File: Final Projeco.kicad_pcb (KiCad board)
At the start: 6 copper layers, 26.5 x 45 mm, 26 parts, among them U1 ESP32-S3, U2 GT-USB-7004N, U3 NCP167BMX330TBG, U4 LY68L6400SLIT, U5 PTS830GG140SMTRLFS, U6 PTS830GG140SMTRLFS, U7 220S-2*16P_H=8_5MM_Ytype_L=3_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, X1 TZ1269D

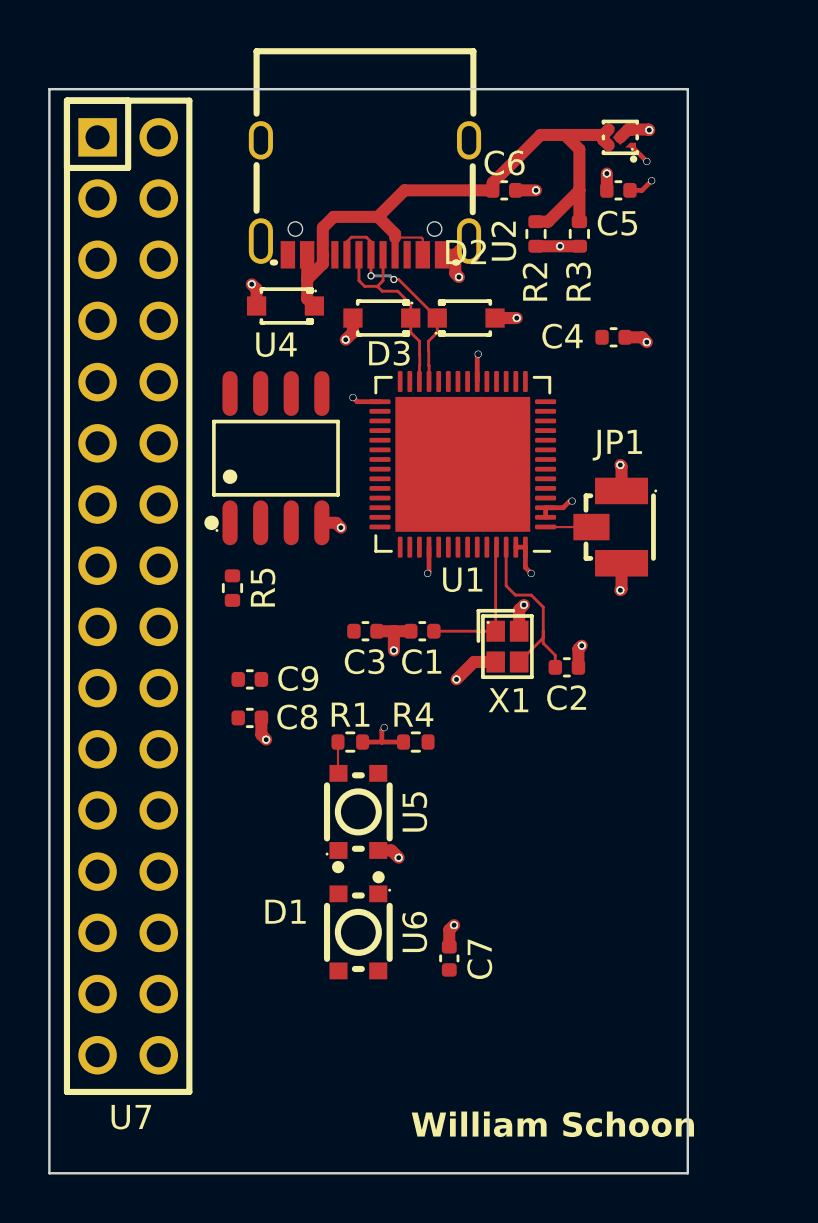
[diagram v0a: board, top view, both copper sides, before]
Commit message: stuff
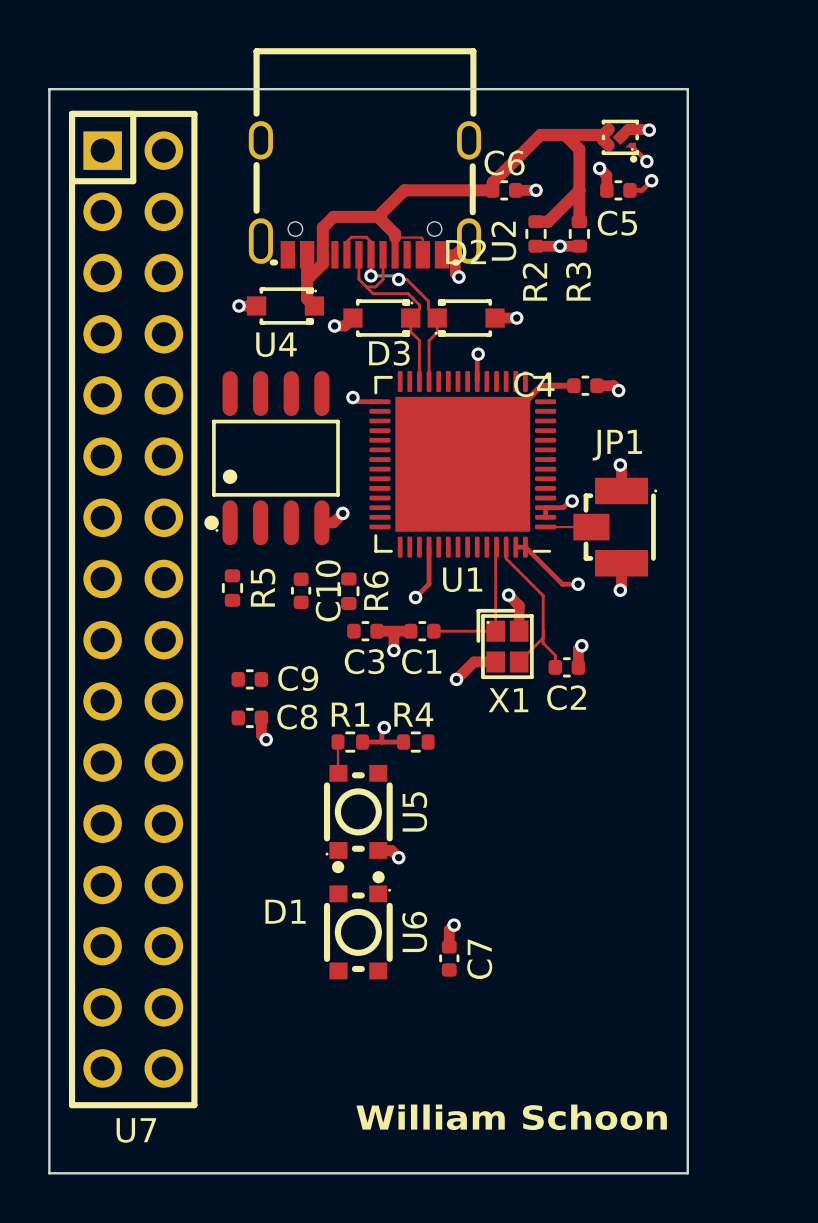
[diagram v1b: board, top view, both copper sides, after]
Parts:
- added C10: 1uF, Capacitor_SMD:C_0402_1005Metric, F.Cu at (35.5, 36.3)
- added R6: 442k, Resistor_SMD:R_0402_1005Metric, F.Cu at (37.4, 36.3)
- C1, C2: value C -> 13pF
- C5, C6: value C -> 1uF
- moved C4 2.33 mm to (47.2, 27.8)
- moved U7 0.59 mm to (28.5, 37.1)
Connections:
- net Net-(U1-GND) renamed /GND_PIN
- U1 pad 37: unconnected-(U1-SPICLK_P/GPIO47-Pad37) -> /SPICLK_GPIO47
- U2 pad 2: unconnected-(U2-SHELL-Pad2) -> GND
- U2 pad 3: unconnected-(U2-SHELL-Pad3) -> GND
- U2 pad 4: unconnected-(U2-SHELL-Pad4) -> GND
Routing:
- net /GND_PIN: track 0.00 -> 5.96 mm
- net VDD3P3: track 11.0 -> 13.9 mm
- net /USB_D-: track 9.03 -> 9.92 mm
- net GND: track 23.2 -> 23.8 mm
